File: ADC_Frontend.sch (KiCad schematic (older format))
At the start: 3 parts

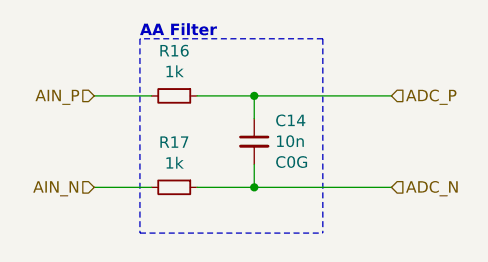
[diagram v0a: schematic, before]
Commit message: PCB Layout Checkpoint
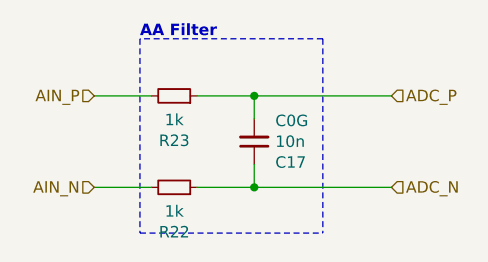
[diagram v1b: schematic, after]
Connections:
- net ADC_N: now also C14.1, R16.1; no longer C14.2, R17.1
- net ADC_P: now also C14.2, R17.1; no longer C14.1, R16.1
- net AIN_N: now also R16.2; no longer R17.2
- net AIN_P: now also R17.2; no longer R16.2
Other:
- moved on the sheet: R22, R23
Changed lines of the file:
@@
 $Descr A4 11693 8268
 encoding utf-8
-Sheet 3 17
+Sheet 6 17
 Title "Kleinvoet"
 Date "2020-06-11"
@@
 Comment4 ""
 $EndDescr
+Wire Notes Line
+	3700 2200 2900 2200
+Text Notes 2900 2200 0    50   ~ 10
+AA Filter
+Text HLabel 2700 2850 0    50   Input ~ 0
+AIN_N
+Text HLabel 2700 2450 0    50   Input ~ 0
+AIN_P
+Text HLabel 4000 2850 2    50   Input ~ 0
+ADC_N
+Text HLabel 4000 2450 2    50   Input ~ 0
+ADC_P
+Wire Notes Line
+	2900 2200 2900 3050
+Wire Notes Line
+	3700 2200 3700 3050
+Wire Notes Line
+	2900 3050 3700 3050
+Connection ~ 3400 2850
+Wire Wire Line
+	4000 2850 3400 2850
+Connection ~ 3400 2450
+Wire Wire Line
+	4000 2450 3400 2450
+Wire Wire Line
+	2700 2450 2950 2450
+Wire Wire Line
+	2700 2850 2950 2850
+Wire Wire Line
+	3400 2450 3400 2550
+Wire Wire Line
+	3150 2450 3400 2450
+Wire Wire Line
+	3400 2850 3400 2750
+Wire Wire Line
+	3150 2850 3400 2850
 $Comp
 L Device:R_Small R?
-U 1 1 5EF8AB51
+U 1 1 5EF8D41D
 P 3050 2450
-AR Path="/5EF8AB51" Ref="R?"  Part="1"
-AR Path="/5EF7F4EB/5EF8AB51" Ref="R?"  Part="1"
-AR Path="/5EFA404B/5EF8AB51" Ref="R?"  Part="1"
-AR Path="/5EFC0F96/5EF8AB51" Ref="R?"  Part="1"
-AR Path="/5EFC2E33/5EF8AB51" Ref="R?"  Part="1"
-AR Path="/5EE5ECAD/5EE62BAF/5EF8AB51" Ref="R16"  Part="1"
-AR Path="/5EE5ECAD/5EE62BB5/5EF8AB51" Ref="R?"  Part="1"
-AR Path="/5EE5ECAD/5EE62BBB/5EF8AB51" Ref="R?"  Part="1"
-AR Path="/5EE5ECAD/5EE62BC1/5EF8AB51" Ref="R?"  Part="1"
-AR Path="/5EE5ECAD/5EE8F492/5EF8AB51" Ref="R18"  Part="1"
-AR Path="/5EE5ECAD/5EE91C90/5EF8AB51" Ref="R20"  Part="1"
-AR Path="/5EE5ECAD/5EE9492B/5EF8AB51" Ref="R22"  Part="1"
-F 0 "R16" V 2854 2450 50  0000 C CNN
+AR Path="/5EF8D41D" Ref="R?"  Part="1"
+AR Path="/5EF7F4EB/5EF8D41D" Ref="R?"  Part="1"
+AR Path="/5EFA404B/5EF8D41D" Ref="R?"  Part="1"
+AR Path="/5EFC0F96/5EF8D41D" Ref="R?"  Part="1"
+AR Path="/5EFC2E33/5EF8D41D" Ref="R?"  Part="1"
+AR Path="/5EE5ECAD/5EE62BAF/5EF8D41D" Ref="R17"  Part="1"
+AR Path="/5EE5ECAD/5EE62BB5/5EF8D41D" Ref="R?"  Part="1"
+AR Path="/5EE5ECAD/5EE62BBB/5EF8D41D" Ref="R?"  Part="1"
+AR Path="/5EE5ECAD/5EE62BC1/5EF8D41D" Ref="R?"  Part="1"
+AR Path="/5EE5ECAD/5EE8F492/5EF8D41D" Ref="R19"  Part="1"
+AR Path="/5EE5ECAD/5EE91C90/5EF8D41D" Ref="R21"  Part="1"
+AR Path="/5EE5ECAD/5EE9492B/5EF8D41D" Ref="R23"  Part="1"
+F 0 "R23" V 2854 2450 50  0000 C CNN
 F 1 "1k" V 2945 2450 50  0000 C CNN
 F 2 "Resistor_SMD:R_0603_1608Metric_Pad1.05x0.95mm_HandSolder" H 3050 2450 50  0001 C CNN
 F 3 "~" H 3050 2450 50  0001 C CNN
-F 4 "ERJ-3RBD102V" V 3050 2450 50  0001 C CNN "MPN"
-F 5 "Panasonic" V 3050 2450 50  0001 C CNN "Mfr."
+F 4 "ERJ-3RBD102V" H 3050 2450 50  0001 C CNN "MPN"
+F 5 "Panasonic" H 3050 2450 50  0001 C CNN "Mfr."
 	1    3050 2450
-	0    1    1    0
+	0    1    -1   0
 $EndComp
 $Comp
@@
 AR Path="/5EE5ECAD/5EE91C90/5EF8AB5E" Ref="C16"  Part="1"
 AR Path="/5EE5ECAD/5EE9492B/5EF8AB5E" Ref="C17"  Part="1"
-F 0 "C14" H 3492 2741 50  0000 L CNN
+F 0 "C17" H 3492 2741 50  0000 L CNN
 F 1 "10n" H 3492 2650 50  0000 L CNN
 F 2 "Capacitor_SMD:C_0603_1608Metric_Pad1.05x0.95mm_HandSolder" H 3400 2650 50  0001 C CNN
@@
 F 6 "KEMET" H 3400 2650 50  0001 C CNN "Mfr."
 	1    3400 2650
-	1    0    0    -1
+	1    0    0    1
 $EndComp
 $Comp
 L Device:R_Small R?
-U 1 1 5EF8D41D
+U 1 1 5EF8AB51
 P 3050 2850
-AR Path="/5EF8D41D" Ref="R?"  Part="1"
-AR Path="/5EF7F4EB/5EF8D41D" Ref="R?"  Part="1"
-AR Path="/5EFA404B/5EF8D41D" Ref="R?"  Part="1"
-AR Path="/5EFC0F96/5EF8D41D" Ref="R?"  Part="1"
-AR Path="/5EFC2E33/5EF8D41D" Ref="R?"  Part="1"
-AR Path="/5EE5ECAD/5EE62BAF/5EF8D41D" Ref="R17"  Part="1"
-AR Path="/5EE5ECAD/5EE62BB5/5EF8D41D" Ref="R?"  Part="1"
-AR Path="/5EE5ECAD/5EE62BBB/5EF8D41D" Ref="R?"  Part="1"
-AR Path="/5EE5ECAD/5EE62BC1/5EF8D41D" Ref="R?"  Part="1"
-AR Path="/5EE5ECAD/5EE8F492/5EF8D41D" Ref="R19"  Part="1"
-AR Path="/5EE5ECAD/5EE91C90/5EF8D41D" Ref="R21"  Part="1"
-AR Path="/5EE5ECAD/5EE9492B/5EF8D41D" Ref="R23"  Part="1"
-F 0 "R17" V 2854 2850 50  0000 C CNN
+AR Path="/5EF8AB51" Ref="R?"  Part="1"
+AR Path="/5EF7F4EB/5EF8AB51" Ref="R?"  Part="1"
+AR Path="/5EFA404B/5EF8AB51" Ref="R?"  Part="1"
+AR Path="/5EFC0F96/5EF8AB51" Ref="R?"  Part="1"
+AR Path="/5EFC2E33/5EF8AB51" Ref="R?"  Part="1"
+AR Path="/5EE5ECAD/5EE62BAF/5EF8AB51" Ref="R16"  Part="1"
+AR Path="/5EE5ECAD/5EE62BB5/5EF8AB51" Ref="R?"  Part="1"
+AR Path="/5EE5ECAD/5EE62BBB/5EF8AB51" Ref="R?"  Part="1"
+AR Path="/5EE5ECAD/5EE62BC1/5EF8AB51" Ref="R?"  Part="1"
+AR Path="/5EE5ECAD/5EE8F492/5EF8AB51" Ref="R18"  Part="1"
+AR Path="/5EE5ECAD/5EE91C90/5EF8AB51" Ref="R20"  Part="1"
+AR Path="/5EE5ECAD/5EE9492B/5EF8AB51" Ref="R22"  Part="1"
+F 0 "R22" V 2854 2850 50  0000 C CNN
 F 1 "1k" V 2945 2850 50  0000 C CNN
 F 2 "Resistor_SMD:R_0603_1608Metric_Pad1.05x0.95mm_HandSolder" H 3050 2850 50  0001 C CNN
 F 3 "~" H 3050 2850 50  0001 C CNN
-F 4 "ERJ-3RBD102V" H 3050 2850 50  0001 C CNN "MPN"
-F 5 "Panasonic" H 3050 2850 50  0001 C CNN "Mfr."
+F 4 "ERJ-3RBD102V" V 3050 2850 50  0001 C CNN "MPN"
+F 5 "Panasonic" V 3050 2850 50  0001 C CNN "Mfr."
 	1    3050 2850
-	0    1    1    0
+	0    1    -1   0
 $EndComp
-Wire Wire Line
-	3150 2450 3400 2450
-Wire Wire Line
-	3400 2450 3400 2550
-Wire Wire Line
-	3150 2850 3400 2850
-Wire Wire Line
-	3400 2850 3400 2750
-Wire Wire Line
-	2700 2450 2950 2450
-Wire Wire Line
-	2700 2850 2950 2850
-Wire Wire Line
-	4000 2850 3400 2850
-Connection ~ 3400 2850
-Wire Wire Line
-	4000 2450 3400 2450
-Connection ~ 3400 2450
-Wire Notes Line
-	2900 3050 3700 3050
-Wire Notes Line
-	3700 2200 2900 2200
-Text Notes 2900 2200 0    50   ~ 10
-AA Filter
-Wire Notes Line
-	3700 2200 3700 3050
-Wire Notes Line
-	2900 2200 2900 3050
-Text HLabel 4000 2450 2    50   Input ~ 0
-ADC_P
-Text HLabel 4000 2850 2    50   Input ~ 0
-ADC_N
-Text HLabel 2700 2450 0    50   Input ~ 0
-AIN_P
-Text HLabel 2700 2850 0    50   Input ~ 0
-AIN_N
 $EndSCHEMATC
